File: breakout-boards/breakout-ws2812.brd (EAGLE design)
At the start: 21.6 x 14 mm, 7 parts

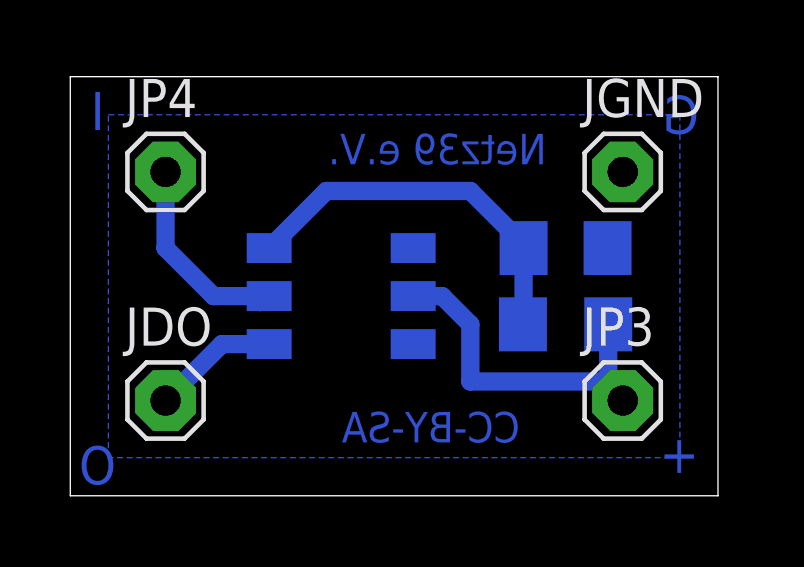
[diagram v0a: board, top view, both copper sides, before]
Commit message: Schönheitskorrekturen
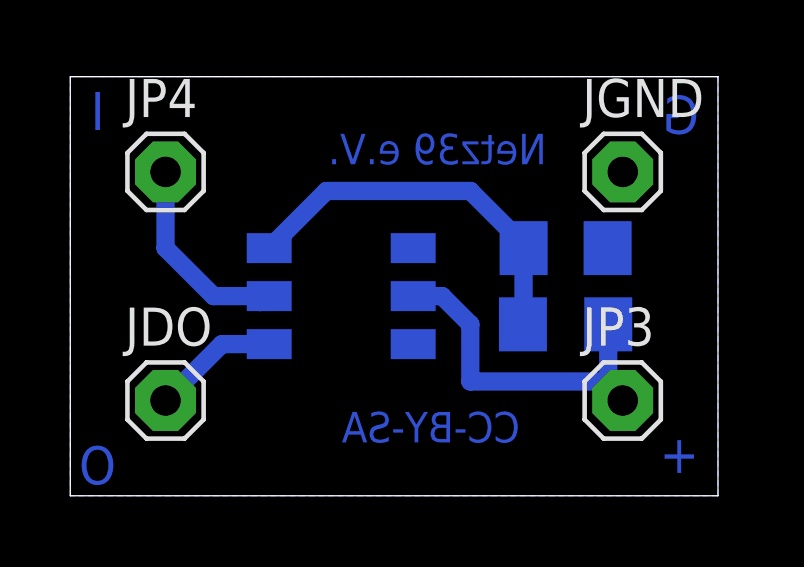
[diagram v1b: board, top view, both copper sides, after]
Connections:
- net JDD renamed VDD
- net N$3 renamed VCC
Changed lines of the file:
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@@
 <setting verticaltext="up"/>
 </settings>
-<grid distance="0.05" unitdist="inch" unit="inch" style="lines" multiple="1" display="yes" altdistance="0.025" altunitdist="inch" altunit="inch"/>
+<grid distance="50" unitdist="mil" unit="mil" style="lines" multiple="1" display="yes" altdistance="25" altunitdist="mil" altunit="mil"/>
 <layers>
 <layer number="1" name="Top" color="4" fill="1" visible="yes" active="yes"/>
@@
 <text x="14.605" y="11.049" size="1.016" layer="16" font="vector" ratio="15" rot="MR0">Netz39 e.V.</text>
 <text x="13.716" y="1.778" size="1.016" layer="16" font="vector" ratio="15" rot="MR0">CC-BY-SA</text>
-<text x="19.685" y="0.762" size="1.27" layer="16" font="vector" rot="MR0">+</text>
-<text x="19.685" y="12.065" size="1.27" layer="16" font="vector" rot="MR0">G</text>
-<text x="0.254" y="0.381" size="1.27" layer="16" font="vector" rot="MR0">O</text>
-<text x="-0.127" y="12.192" size="1.27" layer="16" font="vector" rot="MR0">I</text>
+<text x="19.685" y="0.762" size="1.27" layer="16" font="vector" ratio="15" rot="MR0">+</text>
+<text x="19.685" y="12.065" size="1.27" layer="16" font="vector" ratio="15" rot="MR0">G</text>
+<text x="0.254" y="0.381" size="1.27" layer="16" font="vector" ratio="15" rot="MR0">O</text>
+<text x="-0.127" y="12.192" size="1.27" layer="16" font="vector" ratio="15" rot="MR0">I</text>
 </plain>
 <attributes>
@@
 <signal name="GND">
 <polygon width="0.4064" layer="16">
-<vertex x="0" y="12.7"/>
-<vertex x="19.05" y="12.7"/>
-<vertex x="19.05" y="1.27"/>
-<vertex x="0" y="1.27"/>
+<vertex x="-1.27" y="13.97"/>
+<vertex x="20.32" y="13.97"/>
+<vertex x="20.32" y="0"/>
+<vertex x="-1.27" y="0"/>
 </polygon>
 <contactref element="C1" pad="2"/>
@@
 <contactref element="JGND" pad="1"/>
 </signal>
-<signal name="JDD">
+<signal name="VDD">
 <contactref element="R1" pad="2"/>
 <contactref element="U$1" pad="5"/>
@@
 <wire x1="16.662" y1="3.962" x2="16.662" y2="5.715" width="0.6096" layer="16"/>
 </signal>
-<signal name="N$3">
+<signal name="VCC">
 <contactref element="R1" pad="1"/>
 <contactref element="U$1" pad="3"/>
